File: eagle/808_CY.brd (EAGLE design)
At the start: 100 x 80 mm, 112 parts, among them IC1 TL071P, IC2 TL071P, IC3 TL071P, IC4 TL072P, Q1 2N3904, Q2 2N3904, Q3 2N3904, Q4 2N3904, Q5 2N3904, Q6 2N3904, Q7 2N3904, Q8 2N3906

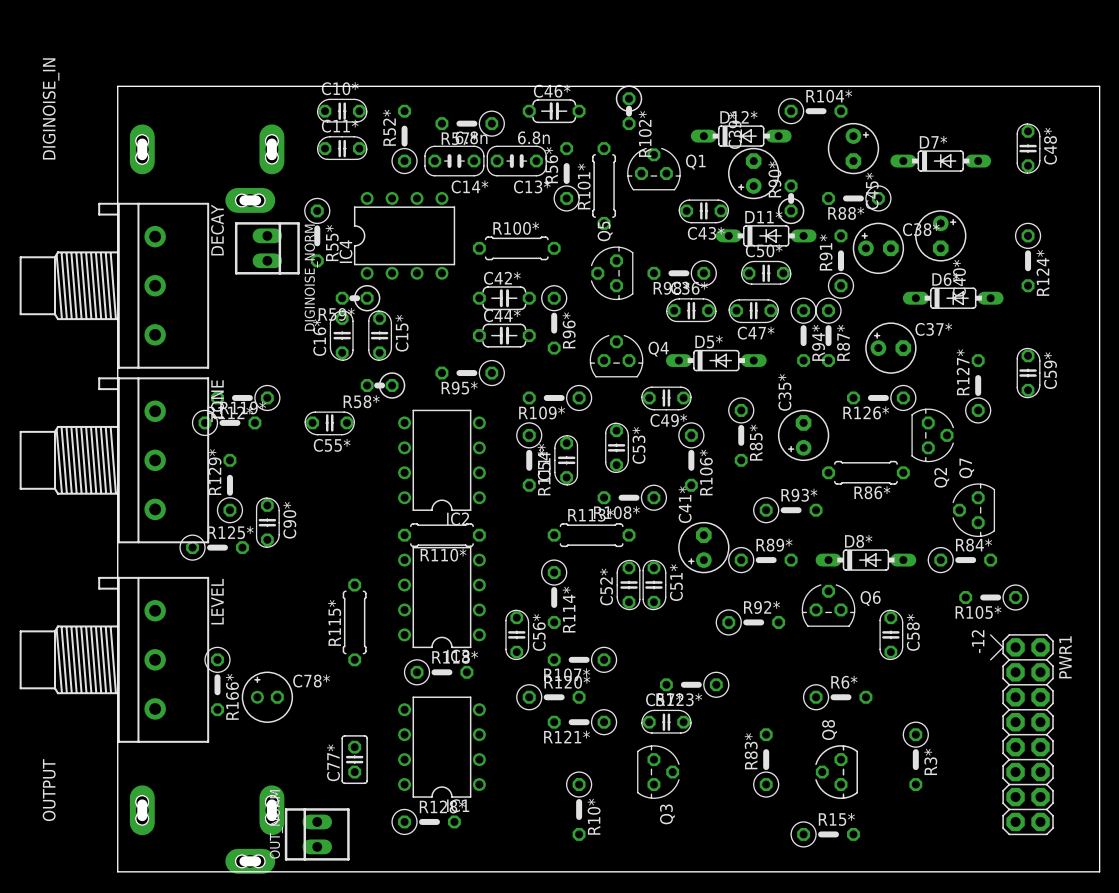
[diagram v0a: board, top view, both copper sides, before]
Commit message: tweaks
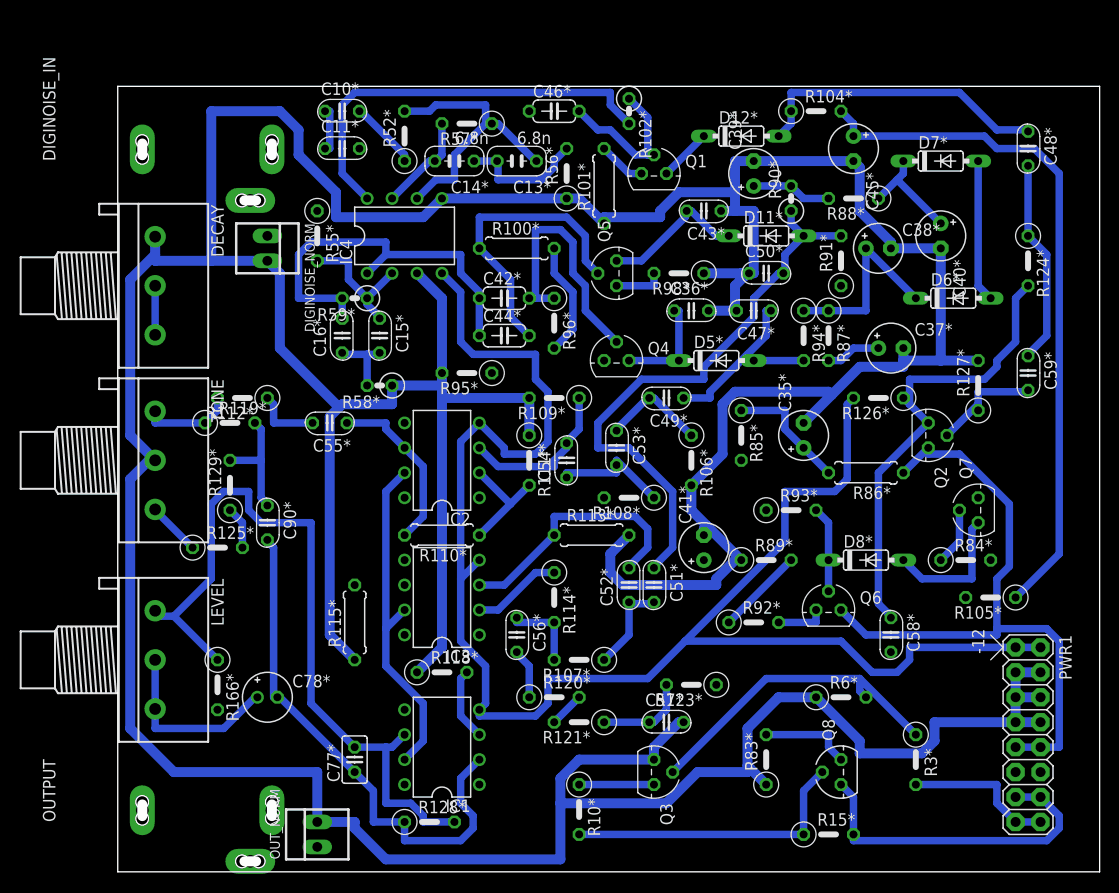
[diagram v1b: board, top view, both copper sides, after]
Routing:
- net GND: track 0.00 -> 549.4 mm
- net -15V: track 0.00 -> 168.9 mm
- net +15V: track 0.00 -> 156.7 mm
- net N$546: track 0.00 -> 79.0 mm
- net N$558: track 0.00 -> 70.6 mm
- net N$223: track 0.00 -> 59.3 mm
- net N$544: track 0.00 -> 54.5 mm
- net N$177: track 0.00 -> 47.6 mm
- net TO_HH: track 0.00 -> 41.0 mm
- net TRIG*: track 0.00 -> 34.2 mm
- net N$517: track 0.00 -> 33.2 mm
- net N$508: track 0.00 -> 30.8 mm
- net N$498: track 0.00 -> 30.1 mm
- net N$516: track 0.00 -> 30.0 mm
- net N$503: track 0.00 -> 28.8 mm
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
